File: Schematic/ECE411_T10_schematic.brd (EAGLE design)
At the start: 100 x 80 mm, 61 parts, among them IC1 LM386MM-1, J1 1, J2 DCJ0202, J3 AVR_SPI_PRG_6PTH, Q1 8.192 MHz, U1 ATMEGA328P_PDIP

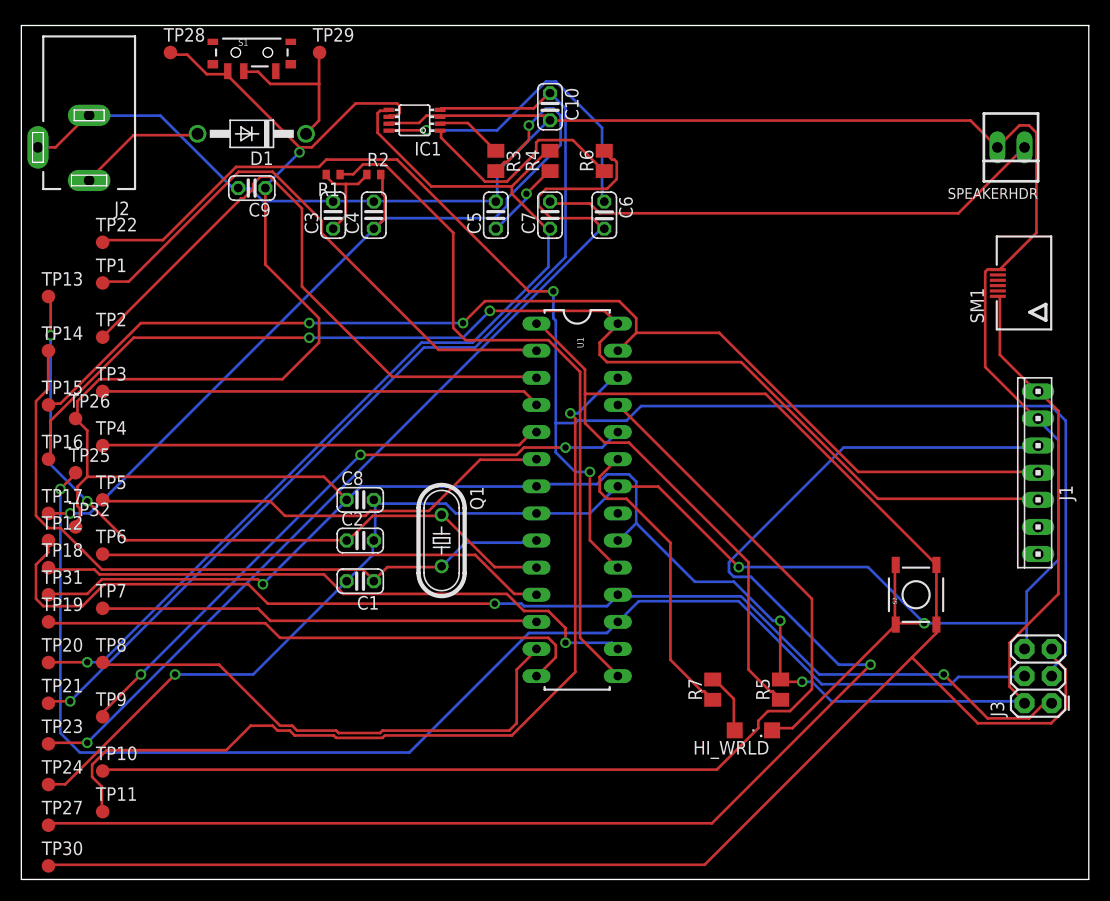
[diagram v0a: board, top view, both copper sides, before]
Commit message: layout preliminary final
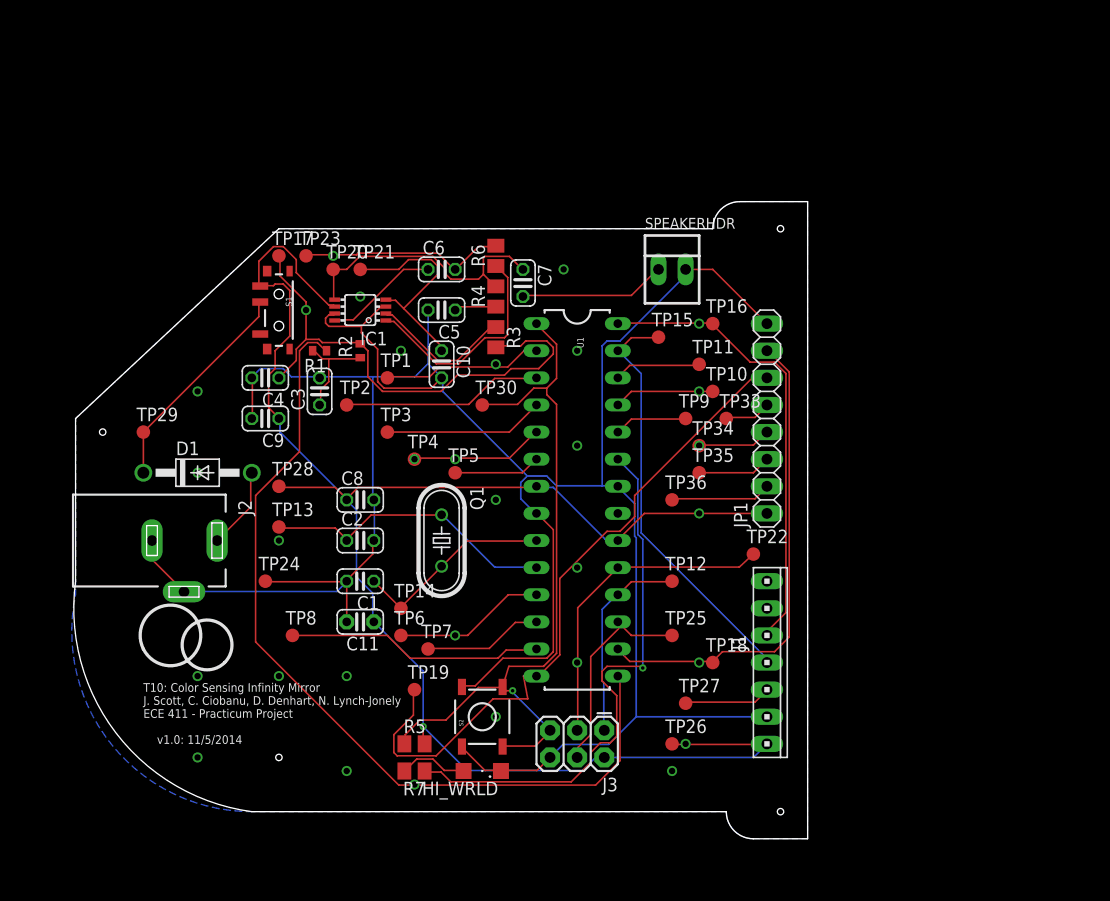
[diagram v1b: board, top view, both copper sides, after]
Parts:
- removed SM1: 06FLZ-SM1, con-jst:6FLZ-SM
- removed TP31, TP32: TPB1,27, testpad:B1,27
- added C11: 100nF, adafruit:C025-024X044
- added JP1: (no value), pinhead:1X08
- added TP33, TP34, TP35, TP36: TPB1,27, testpad:B1,27
- moved TP11 69.9 mm to (63.5, 48.3)
- moved TP22 67.6 mm to (68.6, 30.5)
- moved TP10 67.3 mm to (64.8, 45.7)
- moved TP26 63.7 mm to (61.0, 12.7)
- moved TP16 63.5 mm to (64.8, 52.1)
- moved TP18 62.9 mm to (64.8, 20.3)
- moved TP9 61.3 mm to (62.2, 43.2)
- moved TP27 60.8 mm to (62.2, 16.5)
- moved TP30 59.3 mm to (43.2, 44.5)
- moved TP12 58.5 mm to (61.0, 27.9)
- moved TP25 57.9 mm to (61.0, 22.9)
- moved TP15 57.5 mm to (59.7, 50.8)
- moved TP23 51.7 mm to (26.7, 58.4)
- moved TP21 50.0 mm to (31.8, 57.1)
- moved TP20 45.5 mm to (29.2, 57.1)
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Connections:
- new net N$33: JP1.2, TP36.TP
- new net N$34: JP1.3, TP35.TP
- new net N$35: JP1.4, TP34.TP
- new net N$36: JP1.5, TP33.TP
- net GND: now also C11.2, JP1.8; no longer SM1.6
- net SM1-CLK: now also JP1.6; no longer SM1.3
- net SM1-DAT: now also JP1.7; no longer SM1.5
- net VIN: now also C11.1, JP1.1; no longer SM1.1, TP31.TP, TP32.TP
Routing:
- net RST: track 208.2 -> 69.4 mm, vias 0 -> 1
- net 3.3V: track 134.5 -> 8.17 mm, vias 1 -> 0
- net N$18: track 153.3 -> 30.0 mm, vias 2 -> 0
- net VIN: track 270.9 -> 159.5 mm, vias 4 -> 2
- net N$20: track 125.5 -> 19.8 mm, vias 1 -> 0
- net N$29: track 104.2 -> 9.42 mm, vias 0 -> 1
- net N$19: track 108.9 -> 19.1 mm, vias 2 -> 0
- net N$30: track 84.9 -> 8.17 mm, vias 1 -> 0
- net GND: track 312.9 -> 240.0 mm, vias 3 -> 0
- net N$31: track 92.7 -> 20.6 mm, vias 1 -> 0
- net N$11: track 91.3 -> 19.5 mm, vias 1 -> 0
- net SCL_5.0V: track 111.9 -> 43.1 mm, vias 2 -> 0
- net N$12: track 94.3 -> 26.2 mm, vias 1 -> 0
- net SDA_5.0V: track 106.6 -> 39.3 mm, vias 2 -> 0
- net N$28: track 59.6 -> 6.88 mm, vias 3 -> 0
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- added copper zone on layer 16, net GND
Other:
- board size 100 x 80 mm -> 68.7 x 59.7 mm
- board text added: "T10: Color Sensing Infinity Mirror J. Scott, C. Ciobanu, D. Denhart, N. Lynch-Jonely ECE 411 - Practicum Project v1.0: 11/5/2014"
